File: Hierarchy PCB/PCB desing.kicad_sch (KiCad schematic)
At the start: 39 parts, among them J1 Conn_01x02_Socket, J2 Conn_01x02_Pin, J3 Conn_01x02_Pin, J4 Conn_01x02_Socket, U1 LM2735X, U1 STM32L476RGTx, U1 TPS63001DRC, U2 FGPMMOPA6H, U8 LM386

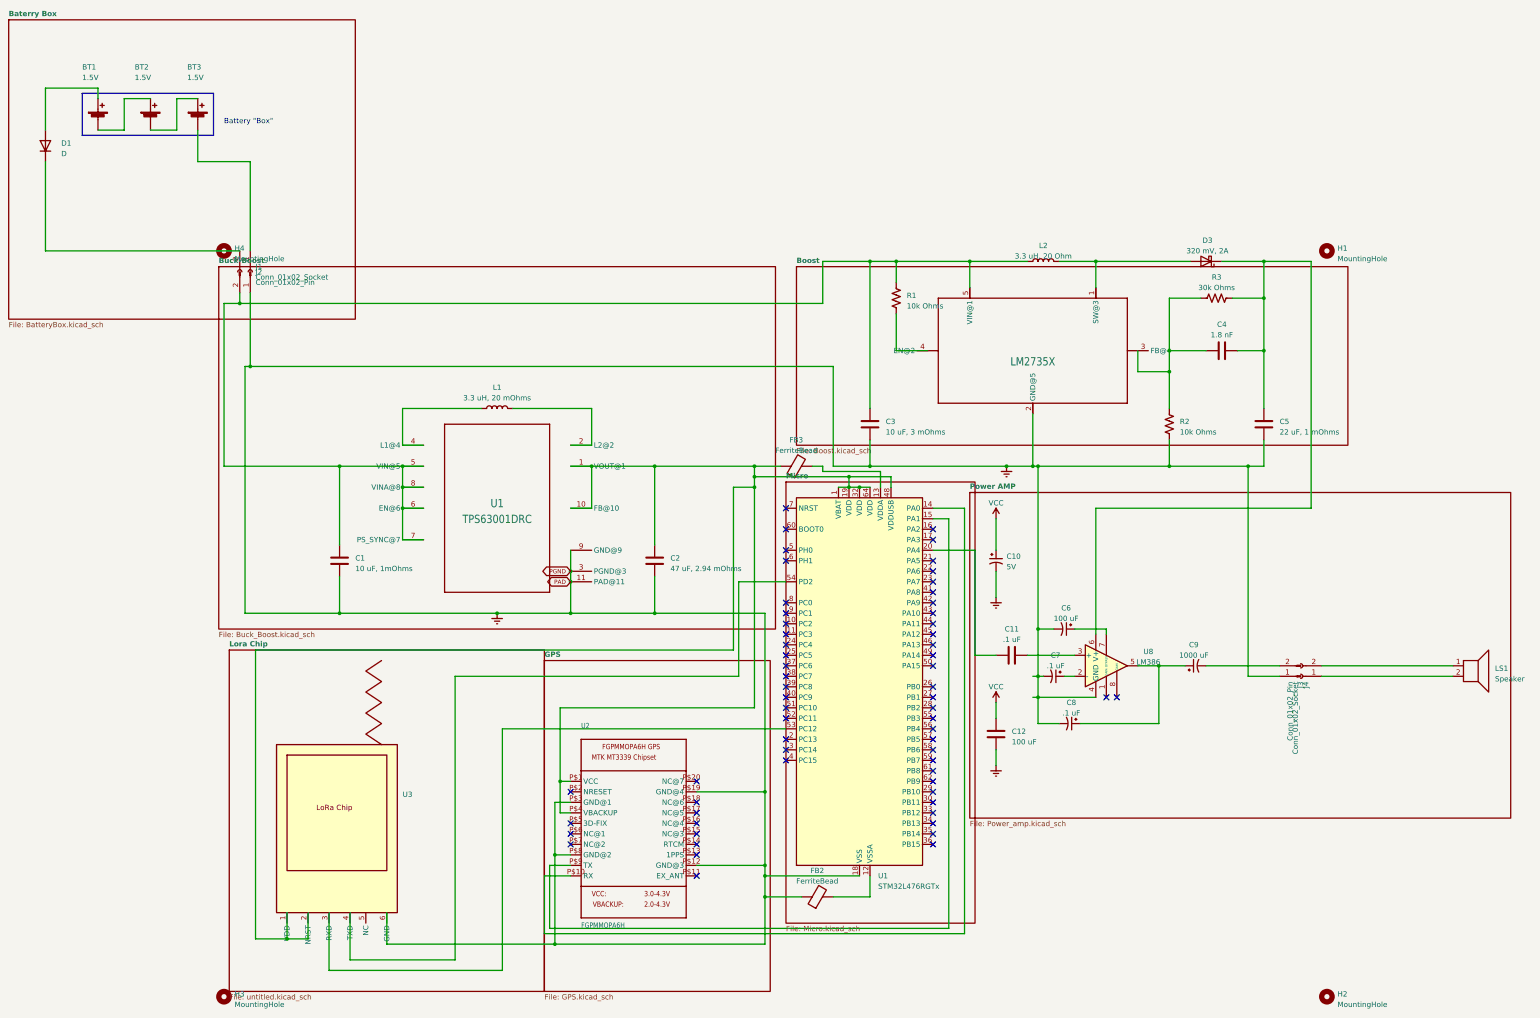
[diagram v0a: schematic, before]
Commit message: Add files via upload
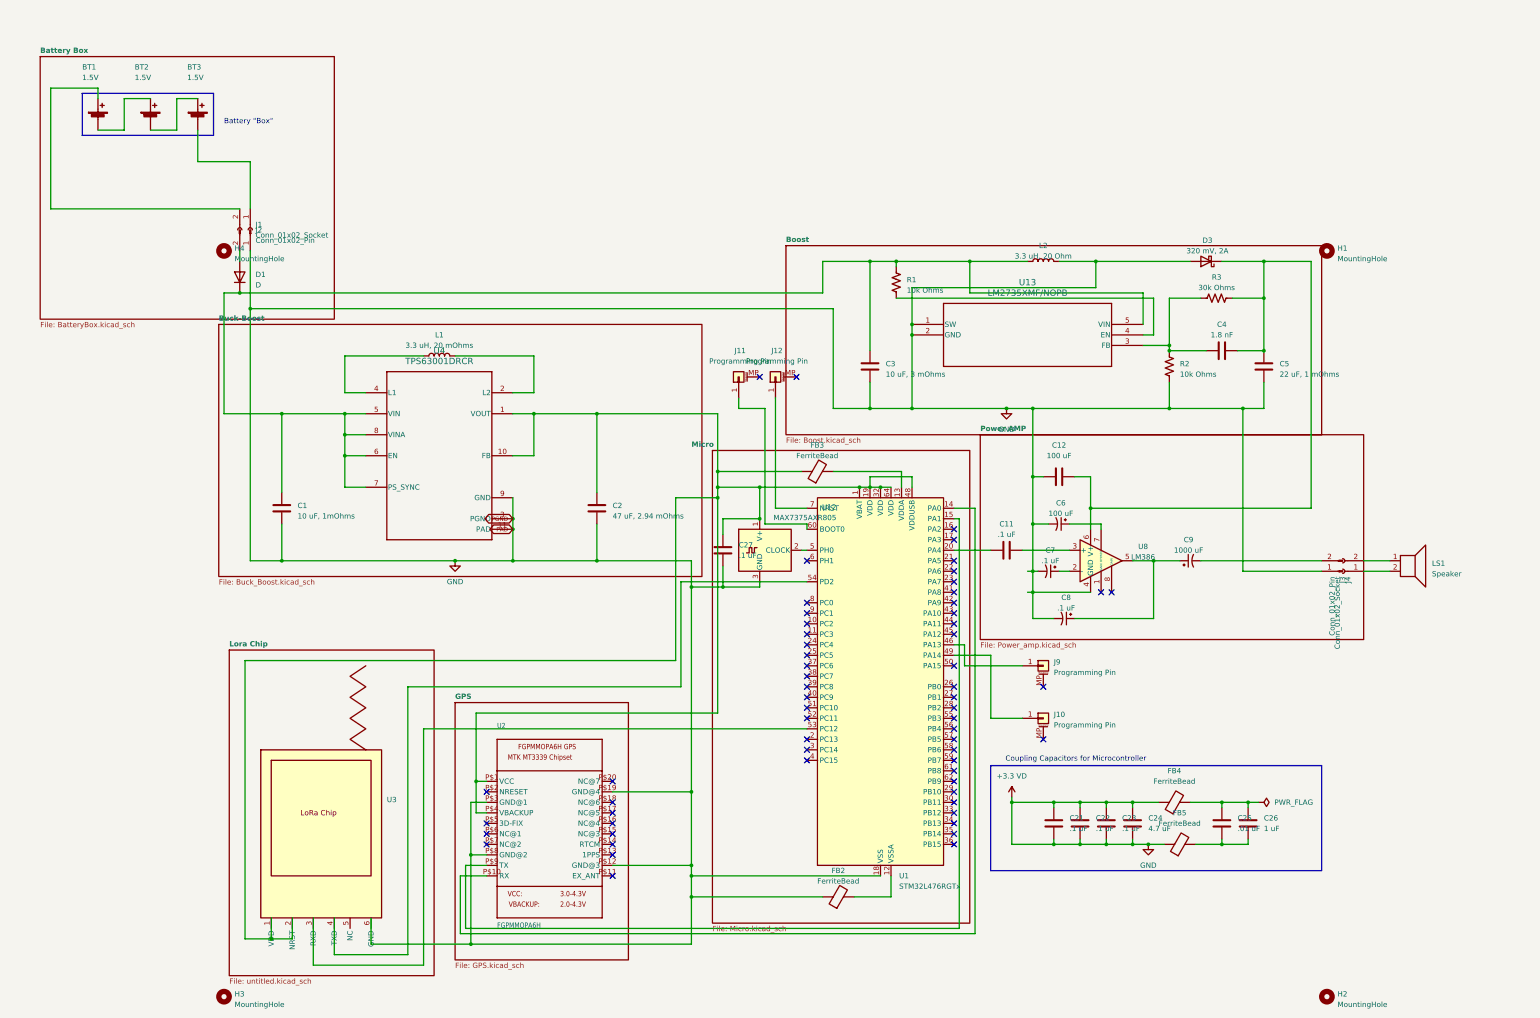
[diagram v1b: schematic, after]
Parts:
- removed C10: 5V, symbol Device:C_Polarized_Small_US
- removed U1: TPS63001DRC, Buck-Boost Converter Chip:DRC0010J, symbol 2024-09-27_13-12-33-eagle-import:TPS63001DRCRTPS63001DRCR
- removed U1: LM2735X, Boost Converter Chip:MF05A, symbol 2024-09-27_13-12-28-eagle-import:LM2735XMF/NOPBLM2735XMF/NOPB
- added C21, C22, C23, C27: .1 uF, symbol Device:C
- added C24: 4.7 uF, symbol Device:C
- added C25: .01 uF, symbol Device:C
- added C26: 1 uF, symbol Device:C
- added FB4, FB5: FerriteBead, symbol Device:FerriteBead
- added J10, J11, J12, J9: Programming Pin, symbol Connector_Generic_MountingPin:Conn_01x01_MountingPin
- added U12: MAX7375AXR805, Package_TO_SOT_SMD:SOT-323_SC-70, symbol Oscillator:MAX7375AXR805
- added U13: LM2735XMF/NOPB, Boost:MF05A, symbol Boost Chip:LM2735XMF_NOPB
- added U4: TPS63001DRCR, Buck-Boost:DRC0010J, symbol Buck-Boost Chip:TPS63001DRCR
- C1, C3, C4, C5: footprint (none) -> Capacitor_SMD:C_0805_2012Metric_Pad1.18x1.45mm_HandSolder
- D1, D3: footprint (none) -> Schottky:Schottky
- FB2, FB3: footprint (none) -> Ferrite_THT:LairdTech_28C0236-0JW-10
- J3: footprint (none) -> Connector_JST:JST_ZH_B2B-ZR-SM4-TF_1x02-1MP_P1.50mm_Vertical
- U8: footprint (none) -> LM386:LM386
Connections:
- net Earth is gone; now on net +3.3 VD: C1.2, C12.1, C2.2, C3.2, C5.2, C6.2, C7.2, C8.2, FB2.1, J2.1 (Pin_1), J3.1 (Pin_1), R2.2, U1.18 (VSS), U1.31 (VSS), U1.47 (VSS), U1.63 (VSS), U2.P$12 (GND@3), U2.P$19 (GND@4), U2.P$3 (GND@1), U2.P$8 (GND@2), U3.6 (GND), U8.4 (GND)
- net VCC is gone; now on an unnamed net: C12.2
- net at C1.1, C3.1, L2.1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: now also D1.1 (K), U13.5 (VIN), U4.5 (VIN), U4.6 (EN), U4.7 (PS_SYNC), U4.8 (VINA); no longer J2.2 (Pin_2)
- net +3.3 VD: now reaches D3.2 (A), L2.2
- net +3.3 VD: now also C21.1, C21.2, C22.1, C22.2, C23.1, C23.2, C24.1, C24.2, C27.2, FB4.1, FB5.1, U12.3 (GND), U13.1 (SW), U13.2 (GND), U4.11 (PAD), U4.3 (PGND), U4.9 (GND)
- net at C2.1, FB3.1, U1.1 (VBAT)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: now also C27.1, U12.1 (V+), U4.1 (VOUT), U4.10 (FB)
- net at L1.2: now also U4.2 (L2)
- net at L1.1: now also U4.4 (L1)
- net at BT1.1 (+): now also J1.2 (Pin_2); no longer D1.2 (A)
- net at U1.46 (PA13): now also J9.1 (Pin_1)
- net at U1.49 (PA14): now also J10.1 (Pin_1)
- net at U1.5 (PH0): now also U12.2 (CLOCK)
- net at U1.60 (BOOT0): now also J11.1 (Pin_1)
- net at U1.7 (NRST): now also J12.1 (Pin_1)
- net at C4.1, R2.1, R3.1: now also U13.3 (FB)
- net at R1.2: now also U13.4 (EN)
- new net: C25.1, C26.1, FB4.2
- new net: C25.2, C26.2, FB5.2
- new net: D1.2 (A), J2.2 (Pin_2)
- no-connect marks 62 -> 61
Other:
- sheet Baterry Box renamed Battery Box
- note added: "Coupling Capacitors for Microcontroller"
- moved on the sheet: C1, C11, C12, C2, C3, C5, C6, C7, C8, C9, FB2, FB3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
